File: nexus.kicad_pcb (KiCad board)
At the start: 2 copper layers, 131.5 x 147.5 mm, 111 parts, among them J1 Screw_Terminal_01x04, J10 Valve_5_PWR, J11 Valve_6_PWR, J12 24V_Lockout_Key_Switch, J13 Ignitor Screw Terminal, J14 PT_1, J15 PT_2, J16 PT_3, J17 PT_4, J18 PT_5, J19 PT_6, J2 Screw_Terminal_01x02, J20 PIN6-9_Breakout, J21 PIN10-13_Breakout, J3 4-Pin Load Cell, J4 5-Pin Load Cell, J5 XT60-M, J6 Valve_1_PWR, J7 Valve_2_PWR, J8 Valve_3_PWR, J9 Valve_4_PWR, K3 G5LE-1, K4 G5LE-1, Q1 BSS138, Q2 BSS138, Q3 BSS138, Q4 BSS138, Q5 BSS138, Q6 BSS138, Q7 BSS138, Q8 BSS138, U1 ESP32-S3, U2 ADS112C04, U3 ADS112C04, U4 ADS112C04, U5 ADS112C04, U6 TPS5430DDA, U7 TPS5430DDA, U8 XC6206P332MR

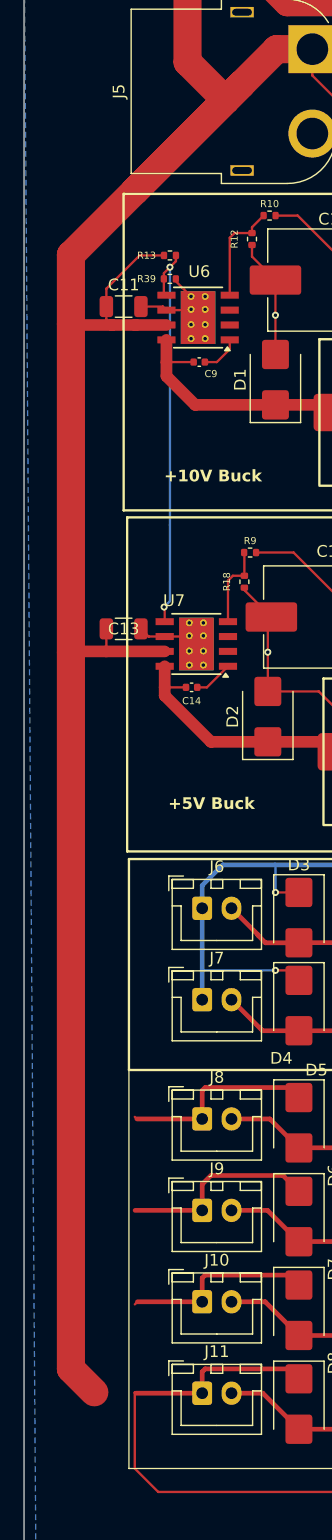
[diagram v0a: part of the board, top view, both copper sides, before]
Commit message: Fix J5
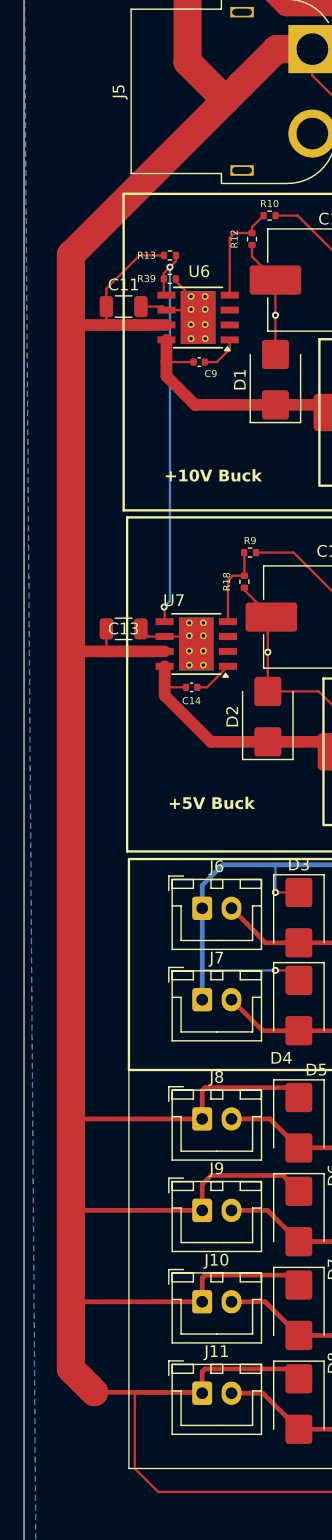
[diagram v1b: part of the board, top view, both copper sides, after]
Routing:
- net +24V: track 390.2 -> 402.9 mm
